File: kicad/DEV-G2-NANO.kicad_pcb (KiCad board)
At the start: 6 copper layers, 76.2 x 20.3 mm, 4 parts, among them U1 MIMXRT1171DVMAB, U2 MAYA-W166-00B

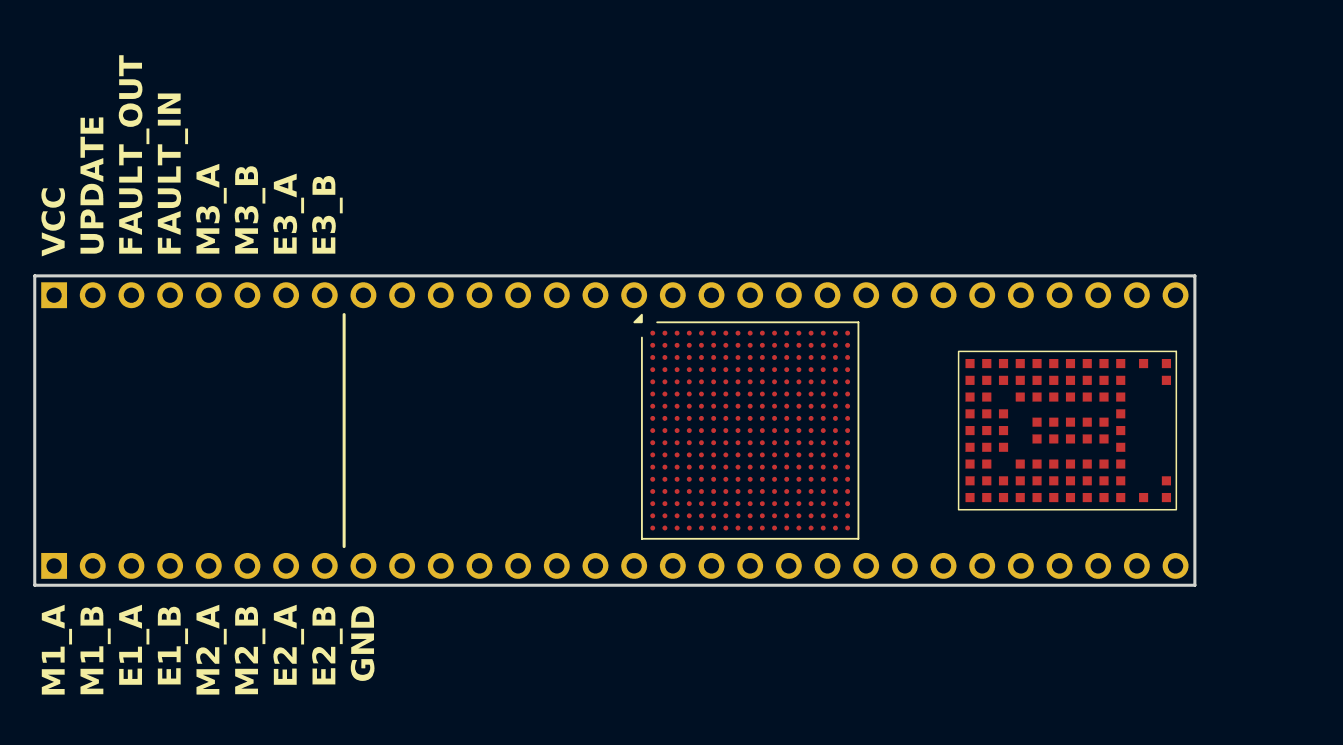
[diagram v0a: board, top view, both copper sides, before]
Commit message: finished preliminary layout
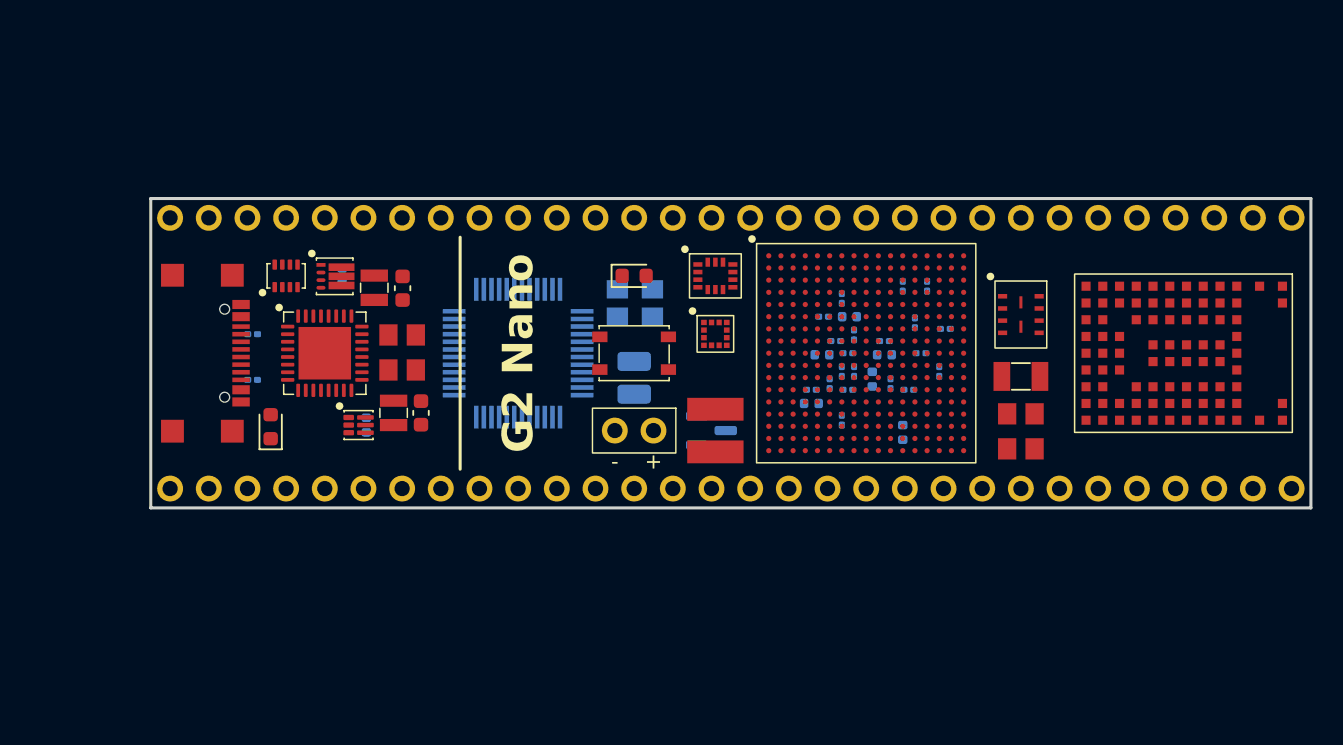
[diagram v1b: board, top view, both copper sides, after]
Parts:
- removed REF** (x2): PinHeader_1x30_P2.54mm_Vertical, Connector_PinHeader_2.54mm:PinHeader_1x30_P2.54mm_Vertical
- added C45: 100nF, Capacitor_SMD:C_0201_0603Metric, B.Cu at (159.0, 97.7)
- added C46: 4.7μF, Capacitor_SMD:C_0402_1005Metric, B.Cu at (159.0, 98.5)
- added C48: 4.7μF, Capacitor_SMD:C_0402_1005Metric, B.Cu at (165.0, 100.5)
- added C49: 1μF, Capacitor_SMD:C_0201_0603Metric, B.Cu at (166.2, 95.2)
- added C50: 2.2μF, Capacitor_SMD:C_0201_0603Metric, B.Cu at (159.8, 92.8)
- added C51: 4.7μF, Capacitor_SMD:C_0402_1005Metric, B.Cu at (161.5, 92.8)
- added C52: 2.2μF, Capacitor_SMD:C_0201_0603Metric, B.Cu at (165.4, 97.7)
- added C57: 100nF, Capacitor_SMD:C_0201_0603Metric, B.Cu at (160.2, 97.2)
- added C58: 2.2μF, Capacitor_SMD:C_0201_0603Metric, B.Cu at (161.4, 97.7)
- added C59: 1μF, Capacitor_SMD:C_0201_0603Metric, B.Cu at (164.2, 97.2)
- added C60: 1μF, Capacitor_SMD:C_0201_0603Metric, B.Cu at (167.4, 96.5)
- added C63: 100nF, Capacitor_SMD:C_0201_0603Metric, B.Cu at (161.0, 96.5)
- added C64: 2.2μF, Capacitor_SMD:C_0201_0603Metric, B.Cu at (161.8, 96.5)
- added C66: 100nF, Capacitor_SMD:C_0201_0603Metric, B.Cu at (161.8, 94.0)
- added C67: 1μF, Capacitor_SMD:C_0201_0603Metric, B.Cu at (163.8, 94.5)
- added C68: 1μF, Capacitor_SMD:C_0201_0603Metric, B.Cu at (161.4, 95.2)
- added C69: 4.7μF, Capacitor_SMD:C_0402_1005Metric, B.Cu at (163.8, 95.3)
- added C70: 4.7μF, Capacitor_SMD:C_0402_1005Metric, B.Cu at (163.0, 97.0)
- added C78: 2.2μF, Capacitor_SMD:C_0201_0603Metric, B.Cu at (166.6, 90.8)
- added C79: 2.2μF, Capacitor_SMD:C_0201_0603Metric, B.Cu at (165.8, 93.2)
- added C80: 2.2μF, Capacitor_SMD:C_0201_0603Metric, B.Cu at (160.6, 94.5)
- added C81: 4.7μF, Capacitor_SMD:C_0402_1005Metric, B.Cu at (159.7, 95.3)
- added C82: 2.2μF, Capacitor_SMD:C_0201_0603Metric, B.Cu at (165.0, 90.8)
- added C83: 2.2μF, Capacitor_SMD:C_0201_0603Metric, B.Cu at (161.0, 91.7)
- added C84: 2.2μF, Capacitor_SMD:C_0201_0603Metric, B.Cu at (161.0, 99.7)
- added C85: 2.2μF, Capacitor_SMD:C_0201_0603Metric, B.Cu at (167.8, 93.7)
- added C86: 10μF, Capacitor_SMD:C_0402_1005Metric, B.Cu at (128.1, 90.2)
- added C87: 22μF, Capacitor_SMD:C_0603_1608Metric, F.Cu at (132.1, 91.0)
- added C89: 4.7μF, Capacitor_SMD:C_0402_1005Metric, B.Cu at (129.7, 100.0)
- added C90: 22μF, Capacitor_SMD:C_0603_1608Metric, F.Cu at (133.3, 99.2)
- added D1: RED, LED_SMD:LED_0603_1608Metric, F.Cu at (147.3, 90.2)
- added D2: BAT54C, project_footprints:BAT54C, B.Cu at (152.4, 100.3)
- added D3: RED, LED_SMD:LED_0603_1608Metric, F.Cu at (123.4, 100.1)
- added J2: Lower Bank, project_footprints:Header-1x30, B.Cu at (116.8, 104.1)
- added J3: Upper Bank, project_footprints:Header-1x30, B.Cu at (190.5, 86.4)
- added J4: USB C, project_footprints:UJ20-C-H-G-SMT-5-P16, F.Cu at (118.1, 95.2)
- added J5: HIC SWD, project_footprints:TestPoints-3, B.Cu at (127.0, 95.2)
- added J6: RTC Battery, project_footprints:Header-1x02, F.Cu at (148.6, 100.3)
- added L1: 10μH, Inductor_SMD:L_1008_2520Metric, B.Cu at (147.3, 96.9)
- added L2: 4.7μH, project_footprints:SDCL1V4018, F.Cu at (152.7, 100.3)
- added L3: 470nH, project_footprints:L_0806, F.Cu at (130.2, 91.0)
- added L4: 470nH, project_footprints:L_0806, F.Cu at (131.5, 99.2)
- added R13: 5.1kΩ, Resistor_SMD:R_0201_0603Metric, B.Cu at (122.3, 94.0)
- added R16: 5.1kΩ, Resistor_SMD:R_0201_0603Metric, B.Cu at (122.3, 97.0)
- added SW1: PTS815, project_footprints:PTS815, F.Cu at (147.3, 95.2)
- added U10: TPS62086, project_footprints:TPS62086, F.Cu at (127.7, 90.2)
- added U11: TPS62825, project_footprints:TPS62825, F.Cu at (129.2, 100.0)
- added U4: LSM6DSV, project_footprints:LSM6DSV, F.Cu at (152.7, 90.2)
- added U5: LIS2MDL, project_footprints:LIS2MDL, F.Cu at (152.7, 94.0)
- added U6: RTMC-G2-4IQ48, project_footprints:RTMC-G2-4IQ48, B.Cu at (139.7, 95.2)
- added U7: W25Q64JWUUIQ, project_footprints:W25Q64JWUUIQ, F.Cu at (172.7, 92.7)
- added U8: MKL26Z128VFM4, project_footprints:MKL26Z128VFM4, F.Cu at (127.0, 95.2)
- added U9: LM66200, project_footprints:LM66200, F.Cu at (124.5, 90.2)
- added Y1: 8MHz, project_footprints:Crystal-4-Pin, B.Cu at (147.3, 91.9)
- added Y2: 16MHz, project_footprints:Crystal-4-Pin, F.Cu at (132.1, 95.2)
- added Y3: 24MHz, project_footprints:Crystal-4-Pin, F.Cu at (172.7, 100.3)
- added Y4: 32.768kHz, project_footprints:Crystal-2-Pin, F.Cu at (172.7, 96.8)
- U2: renamed from U1; footprint Package_BGA:MAPBGA-289_14x14mm_Layout17x17_P0.8mm -> project_footprints:MIMXRT1171DVMAB
- moved U2 9.16 mm to (162.6, 95.2)
- moved U3 9.16 mm to (183.6, 95.2)
- renumbered U2 to U3
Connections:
- U2 pad D17: Net-(J1-Pin_1) -> +5V
- U2 pad G12: +3V3 -> Net-(U2A-VDD_USB_3P3)
- U2 pad G16: V_{DCDC_ANA} -> +1V8
- U2 pad H12: V_{DCDC_ANA} -> Net-(U2A-VDD_USB_1P8)
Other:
- board text added: "+"
- board text added: "-"
- board text added: "G2 Nano"
- board text added: "VIN (+5V)"
- board text removed: "E1_A"
- board text removed: "E1_B"
- board text removed: "E2_A"
- board text removed: "E2_B"
- board text removed: "E3_A"
- board text removed: "E3_B"
- board text removed: "FAULT_IN"
- board text removed: "FAULT_OUT"
- board text removed: "M1_A"
- board text removed: "M1_B"
- board text removed: "M2_A"
- board text removed: "M2_B"
- board text removed: "M3_A"
- board text removed: "M3_B"
- board text removed: "UPDATE"
- board text removed: "VCC"
